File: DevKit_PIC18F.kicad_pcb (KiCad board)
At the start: 2 copper layers, 40 x 69 mm, 27 parts, among them J1 PIC_ICSP_ICD, J2 USB_C_Receptacle_USB2.0_16P, J4 RA_PORT, J5 RB_PORT, J6 RD_PORT, J7 RC_PORT, J8 RE_PORT, J9 2P_UART, SW1 SW_DIP, X1 16MHz

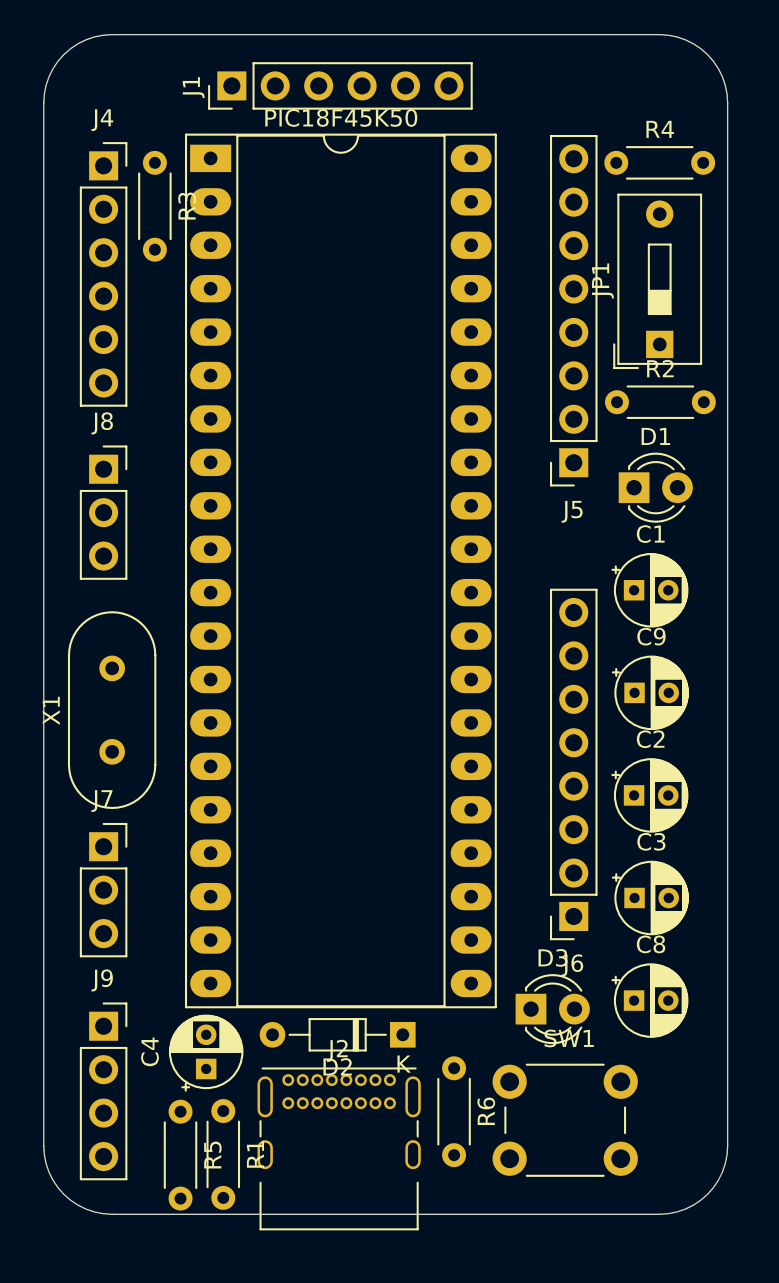
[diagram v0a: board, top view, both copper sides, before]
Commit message: Routed & Finished Rev.1
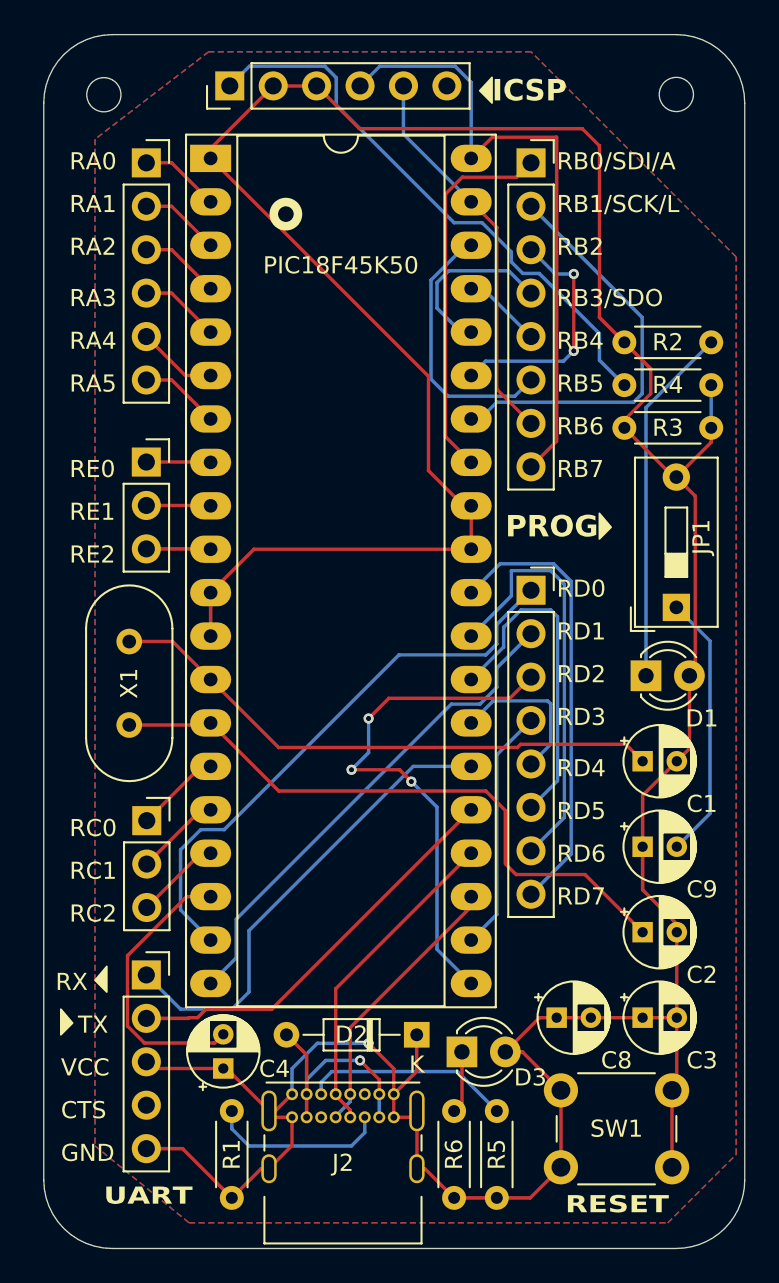
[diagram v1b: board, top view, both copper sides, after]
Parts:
- J9: footprint Connector_PinSocket_2.54mm:PinSocket_1x04_P2.54mm_Vertical -> Connector_PinSocket_2.54mm:PinSocket_1x05_P2.54mm_Vertical
- moved R3 31.5 mm to (102.0, 49.5), turned to 0 degrees
- moved J6 19.2 mm to (96.5, 59.0), turned to 0 degrees
- moved R5 18.5 mm to (94.5, 89.5)
- moved J5 17.7 mm to (96.5, 34.0), turned to 0 degrees
- moved JP1 15.4 mm to (105.0, 60.0)
- moved R4 13.0 mm to (102.0, 47.0)
- moved D1 11.0 mm to (103.2, 64.0)
- moved C1 10.0 mm to (103.0, 69.0)
- moved C9 9.01 mm to (103.0, 74.0)
- moved C2 8.02 mm to (103.0, 79.0)
- moved C3 7.02 mm to (103.0, 84.0)
- moved R2 6.53 mm to (107.0, 44.5), turned to 180 degrees
- moved D3 4.75 mm to (92.5, 86.0)
- moved C8 4.64 mm to (98.0, 84.0)
- moved J9 3.91 mm to (74.0, 81.5)
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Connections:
- J5 pad 7: /PGD -> /PGC
- J5 pad 8: /PGC -> /PGD
- J9 pad 4: GND -> unconnected-(J9-Pin_4-Pad4)
- PIC18F45K50 pad 39: /PGD -> /PGC
- PIC18F45K50 pad 40: /PGC -> /PGD
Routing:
- net GND: track 0.00 -> 220.5 mm, vias 0 -> 1
- net /PGD: track 0.00 -> 37.2 mm
- net /OSC2: track 0.00 -> 37.0 mm
- net Net-(J6-Pin_1): track 0.00 -> 33.5 mm
- net /MCLR: track 0.00 -> 33.5 mm
- net /OSC1: track 0.00 -> 33.1 mm
- net Net-(J6-Pin_3): track 0.00 -> 31.0 mm, vias 0 -> 3
- net Net-(J6-Pin_2): track 0.00 -> 29.2 mm
- net Net-(J9-Pin_1): track 0.00 -> 27.8 mm
- net Net-(J6-Pin_8): track 0.00 -> 26.2 mm
- net Net-(J6-Pin_7): track 0.00 -> 24.6 mm
- net Net-(J5-Pin_2): track 0.00 -> 24.3 mm
- net Net-(J9-Pin_2): track 0.00 -> 24.1 mm
- net /PGC: track 0.00 -> 22.8 mm
- net Net-(J5-Pin_1): track 0.00 -> 22.1 mm
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- added copper zone on B.Cu, net (none)
- added copper zone on F.Cu, net (none)
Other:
- board size 40 x 69 mm -> 41 x 71 mm
- board text added: "CTS"
- board text added: "GND"
- board text added: "ICSP"
- board text added: "PROG"
- board text added: "RA0"
- board text added: "RA1"
- board text added: "RA2"
- board text added: "RA3"
- board text added: "RA4"
- board text added: "RA5"
- board text added: "RB0/SDI/A"
- board text added: "RB1/SCK/L"
- board text added: "RB2"
- board text added: "RB3/SDO"
- board text added: "RB4"
- board text added: "RB5"
- board text added: "RB6"
- board text added: "RB7"
- board text added: "RC0"
- board text added: "RC1"
- board text added: "RC2"
- board text added: "RD0"
- board text added: "RD1"
- board text added: "RD2"
- board text added: "RD3"
- board text added: "RD4"
- board text added: "RD5"
- board text added: "RD6"
- board text added: "RD7"
- board text added: "RE0"
- board text added: "RE1"
- board text added: "RE2"
- board text added: "RESET"
- board text added: "RX"
- board text added: "TX"
- board text added: "UART"
- board text added: "VCC"
